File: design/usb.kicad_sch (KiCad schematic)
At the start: 27 parts, among them J4 USB_B_Mini, SW1 RST, U7 USBLC6-2SC6, U8 SN74LVC1G11DCKR, U9 FT231XS

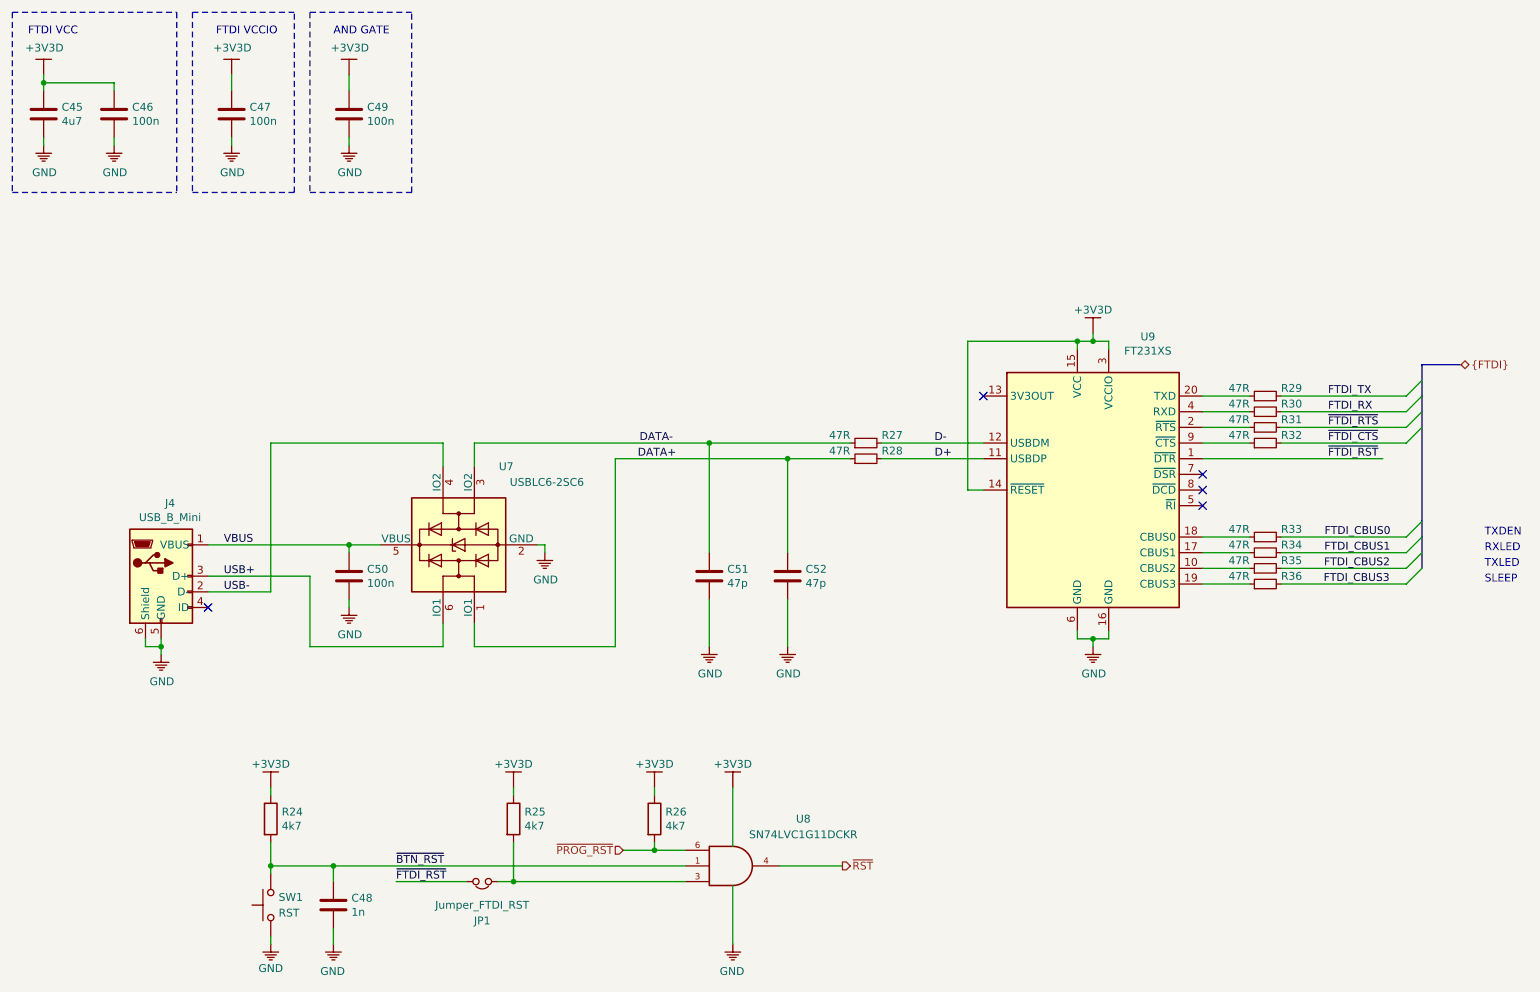
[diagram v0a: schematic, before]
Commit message: Updated notes
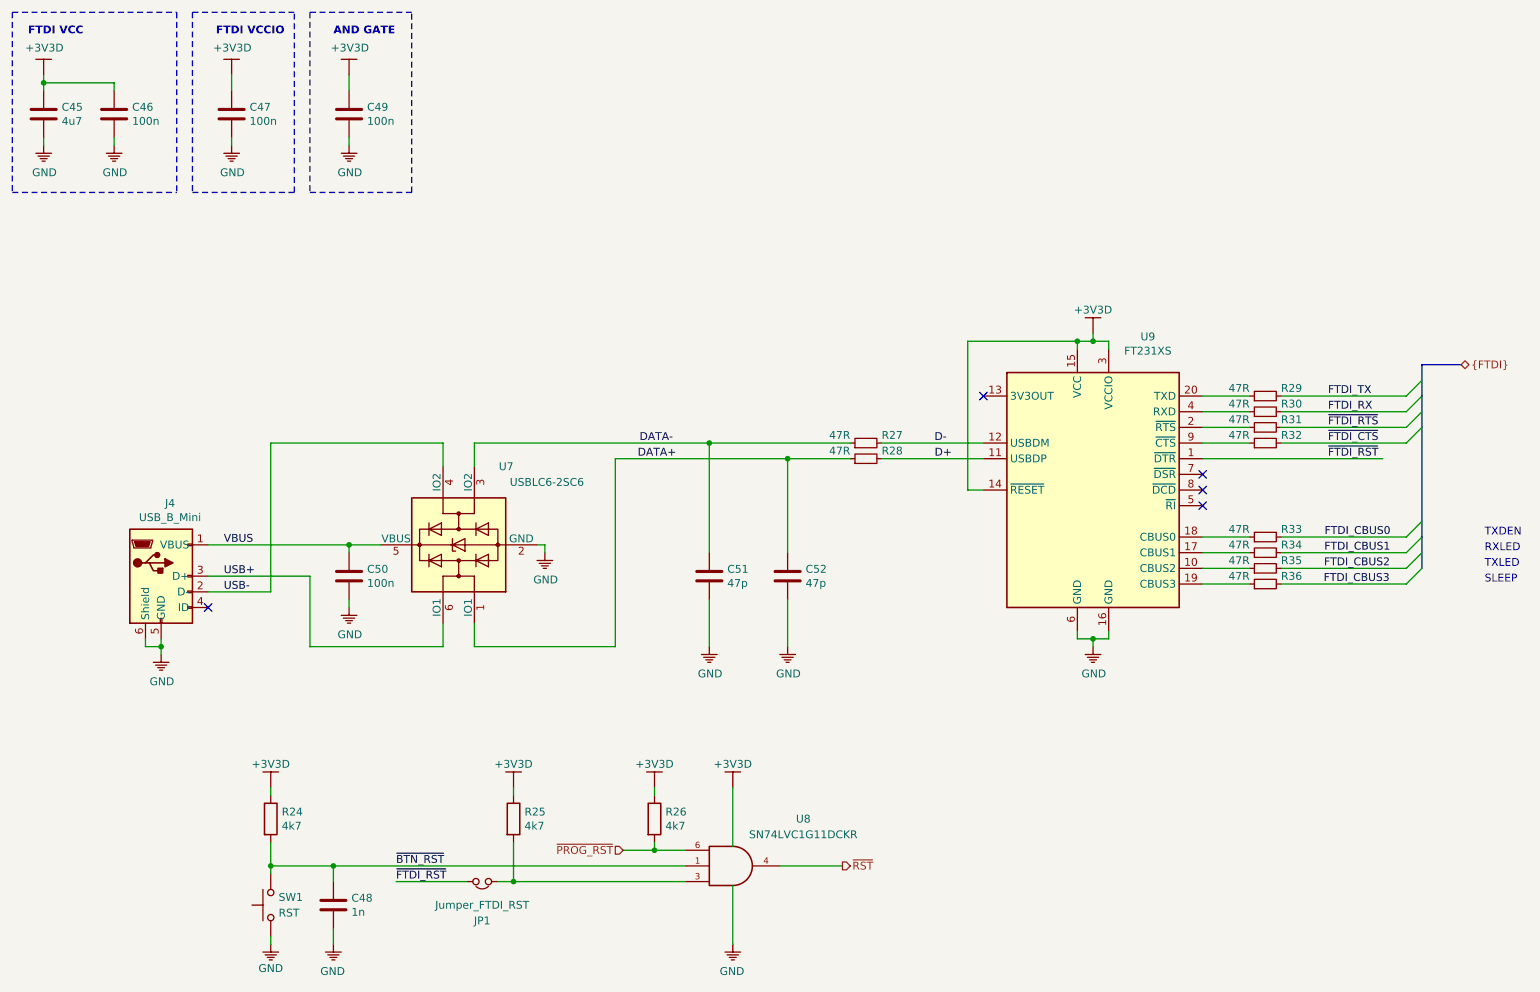
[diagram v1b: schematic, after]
